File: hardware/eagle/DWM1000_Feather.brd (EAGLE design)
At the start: 59.7 x 22.9 mm, 42 parts, among them J1 DX07B024JJ3R1600, J4 20021221-00010C4LF, SW1 SPST_TACT-KMR2, U1 ATSAMD21G-M, U2 MCP73831, U3 DWM1000, U4 AP2112K-3.3TRG1, Y1 FC-135_32.7680KA-A0

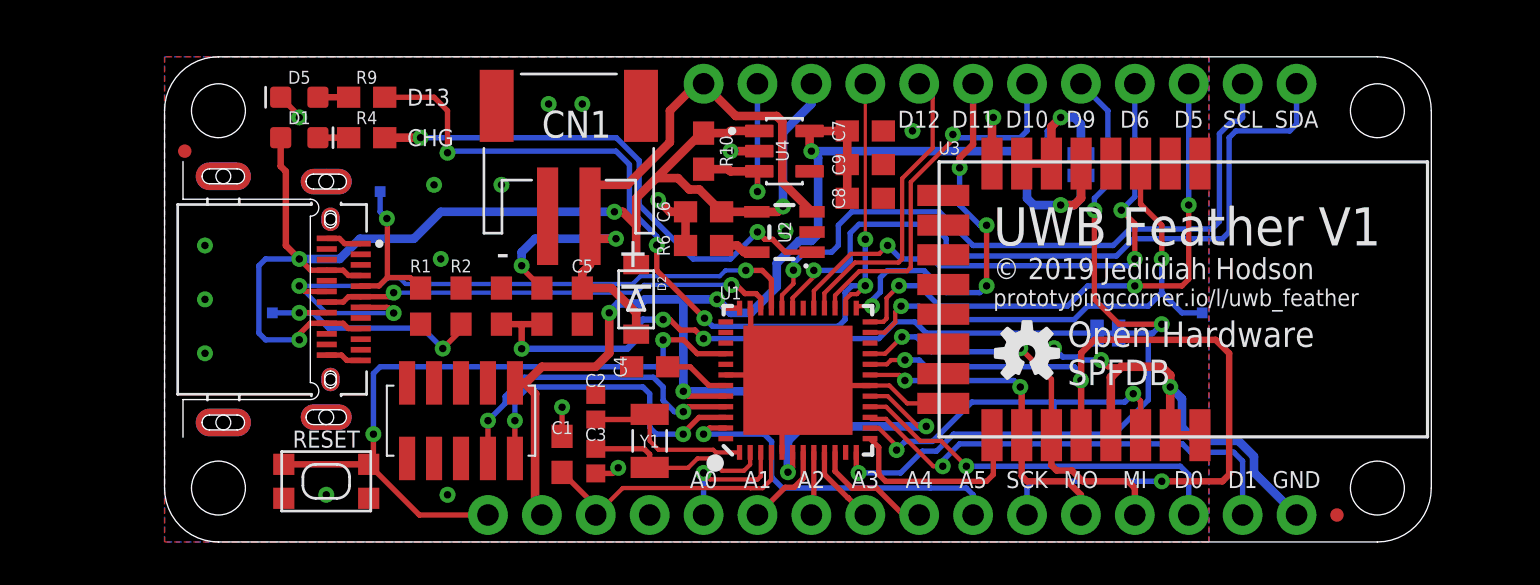
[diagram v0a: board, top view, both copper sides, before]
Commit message: Version 1.1 update. BRD is INCOMPLETE
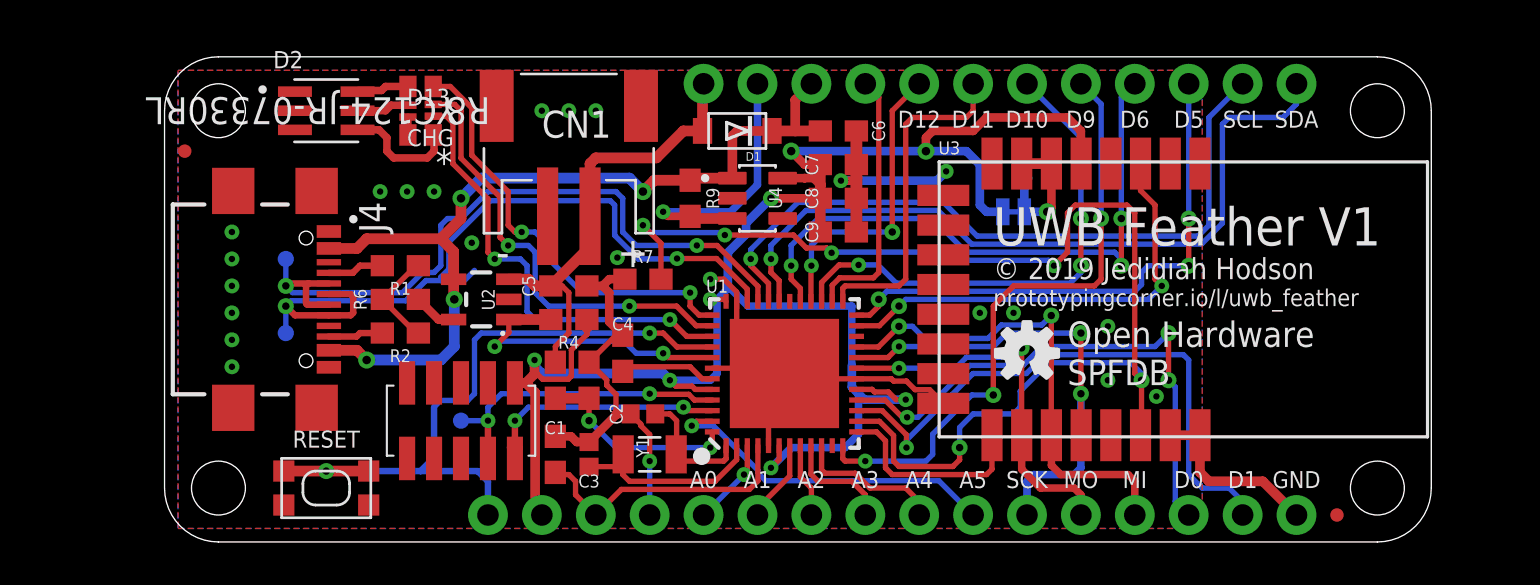
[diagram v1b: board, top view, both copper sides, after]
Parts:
- removed D5: BLUE, SparkFun-LED:LED-0603
- removed J1: DX07B024JJ3R1600, DX07B024JJ3R1600:JAE_DX07B024JJ3R1600
- removed R10: 10K, SparkFun-Resistors:0603
- removed TP6: TEST-POINT2, SparkFun-Connectors:PAD.02X.02
- added R7: 100K, SparkFun-Resistors:0603
- added R8: YC124-JR-07330RL, YC124-JR-07330RL:YAG_YC124
- added TP2: TEST-POINT3, SparkFun-Connectors:PAD.03X.03
- D1: value ORANGE -> (none); device SparkFun-LED:LED-0603 -> adafruit:SOD-123FL
- D2: value (none) -> ASMT-YTD7-0AA02; device adafruit:SOD-123FL -> ASMT-YTD7-0AA02:LED_ASMT-YTD7-0AA02
- J4: value 20021221-00010C4LF -> USB4110-GF-A; device 20021221-00010C4LF:20021221-00010C4LF -> USB4110-GF-A:GCT_USB4110-GF-A
- JP1: value BATT_DETECT -> DWM_3V3
- JP2: value DWM_3V3 -> 20021221-00010C4LF; device SparkFun-Jumpers:SMT-JUMPER_2_NC_TRACE_SILK -> 20021221-00010C4LF:20021221-00010C4LF
- R4: value 1K -> 5K1
- R9: value 330 -> 10K
- TP1, TP3, TP4, TP5: value TEST-POINT2 -> TEST-POINT3; device SparkFun-Connectors:PAD.02X.02 -> SparkFun-Connectors:PAD.03X.03
- U2: value MCP73831 -> MCP73832
- moved TP1 36.9 mm to (5.71, 9.84), turned to 0 degrees
- moved JP2 31.6 mm to (14.0, 5.71), flipped to the top, turned to 180 degrees
- moved D1 20.6 mm to (27.0, 19.4), turned to 180 degrees
- moved D2 17.1 mm to (7.62, 20.3), turned to 0 degrees
- moved R9 16.0 mm to (24.8, 16.2), turned to 270 degrees
- moved U2 14.6 mm to (14.9, 11.4)
- moved R6 14.5 mm to (11.1, 11.4)
- moved TP3 13.6 mm to (16.5, 4.45), turned to 0 degrees
- moved R4 12.8 mm to (19.1, 10.5), turned to 180 degrees
- moved TP5 10.5 mm to (40.5, 17.1), turned to 0 degrees
- moved TP4 10.2 mm to (14.0, 5.71), turned to 0 degrees
- moved J4 9.27 mm to (6.67, 11.4), turned to 270 degrees
- moved C6 7.41 mm to (31.8, 19.4), turned to 0 degrees
- moved JP1 7.24 mm to (40.0, 15.6), turned to 0 degrees
- moved R3 4.32 mm to (18.4, 7.62)
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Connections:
- removed net CC1: J1.A5, R1.2, TP3.P$1
- removed net CC2: J1.B5, R2.2, TP4.P$1
- removed net DWM_WU: U3.2
- removed net N$9: D5.A, R9.1
- removed net RX_LED: U3.13
- removed net TX_LED: U3.12
- new net BATT_S: R4.2, U1.41, U2.1
- new net BATT_V: R3.2, R5.1, U1.48
- new net N$1: D2.6, R8.5
- new net N$10: J4.B5, R2.2
- new net N$8: J4.A5, R1.2
- new net RGB_B: R8.4, U1.37
- new net RGB_G: R8.3, U1.38
- new net RGB_R: R8.2, U1.39
- net 3.3V: now also JP1.2, JP2.1, R4.1; no longer J4.1, JP2.2
- net D+: now also J4.A6, J4.B6, TP1.P$1; no longer J1.A6, J1.B6
- net D-: now also J4.A7, J4.B7, TP2.P$1; no longer J1.A7, J1.B7
- net D13: no longer R9.2
- net D2: no longer TP5.P$1
- net D3: now also R7.2; no longer TP6.P$1
- net D9: no longer JP1.2
- net DWM_3V3: now also JP1.1, TP5.P$1; no longer JP2.1, TP1.P$1
- net EN: now also R9.2; no longer R10.2
- net GND: now also D2.1, D2.2, D2.3, J4.A1/B12, J4.B1/A12, J4.S1, J4.S2, J4.S3, J4.S4, JP2.3, JP2.5, JP2.9, R5.2, R7.1; no longer D5.C, J1.A1, J1.A12, J1.B1, J1.B12, J1.S1, J1.S2, J1.S3, J1.S4, J1.S5, J1.S6, J4.3, J4.5, J4.9, R3.1
- net N$3: now also D2.5, R8.6; no longer D1.C, R4.1
- net N$4: now also R8.7, R8.8; no longer R4.2, U2.1
- net N$5: now also D2.4, R8.1; no longer JP1.1, R3.2, R5.1
- net SWCLK: now also JP2.4, TP4.P$1; no longer J4.4
- net SWDIO: now also JP2.2, TP3.P$1; no longer J4.2
- net V_BATT: now also D1.A, R3.1; no longer D2.A, R5.2
- net V_USB: now also D1.C, J4.A4/B9, J4.B4/A9, R9.1; no longer D1.A, D2.C, J1.A4, J1.A9, J1.B4, J1.B9, R10.1
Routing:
- net D3: track 17.0 -> 58.8 mm, vias 2 -> 6
- net D13: track 43.2 -> 12.4 mm, vias 5 -> 0
- net N$5: track 32.0 -> 5.43 mm, vias 3 -> 0
- net N$4: track 24.6 -> 0.84 mm, vias 2 -> 0
- net RGB_R: track 0.00 -> 21.3 mm, vias 0 -> 2
- net RGB_G: track 0.00 -> 21.0 mm, vias 0 -> 2
- net RGB_B: track 0.00 -> 20.6 mm, vias 0 -> 2
- net V_USB: track 60.4 -> 41.9 mm
- net SCK: track 38.8 -> 23.7 mm
- net D+: track 21.5 -> 36.2 mm
- net BATT_S: track 0.00 -> 14.2 mm, vias 0 -> 2
- net V_BATT: track 34.6 -> 21.6 mm, vias 2 -> 0
- net CC2: track 11.5 -> 0.00 mm, vias 2 -> 0
- net BATT_V: track 0.00 -> 9.66 mm, vias 0 -> 2
- net 3.3V: track 82.0 -> 90.3 mm, vias 7 -> 8
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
